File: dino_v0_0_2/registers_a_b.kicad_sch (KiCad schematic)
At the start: 8 parts, among them U31 74LS373, U32 74LS373, U33 74LS373, U35 74LS373, U41 74LS245, U42 74LS245, U43 74LS245, U44 74LS245

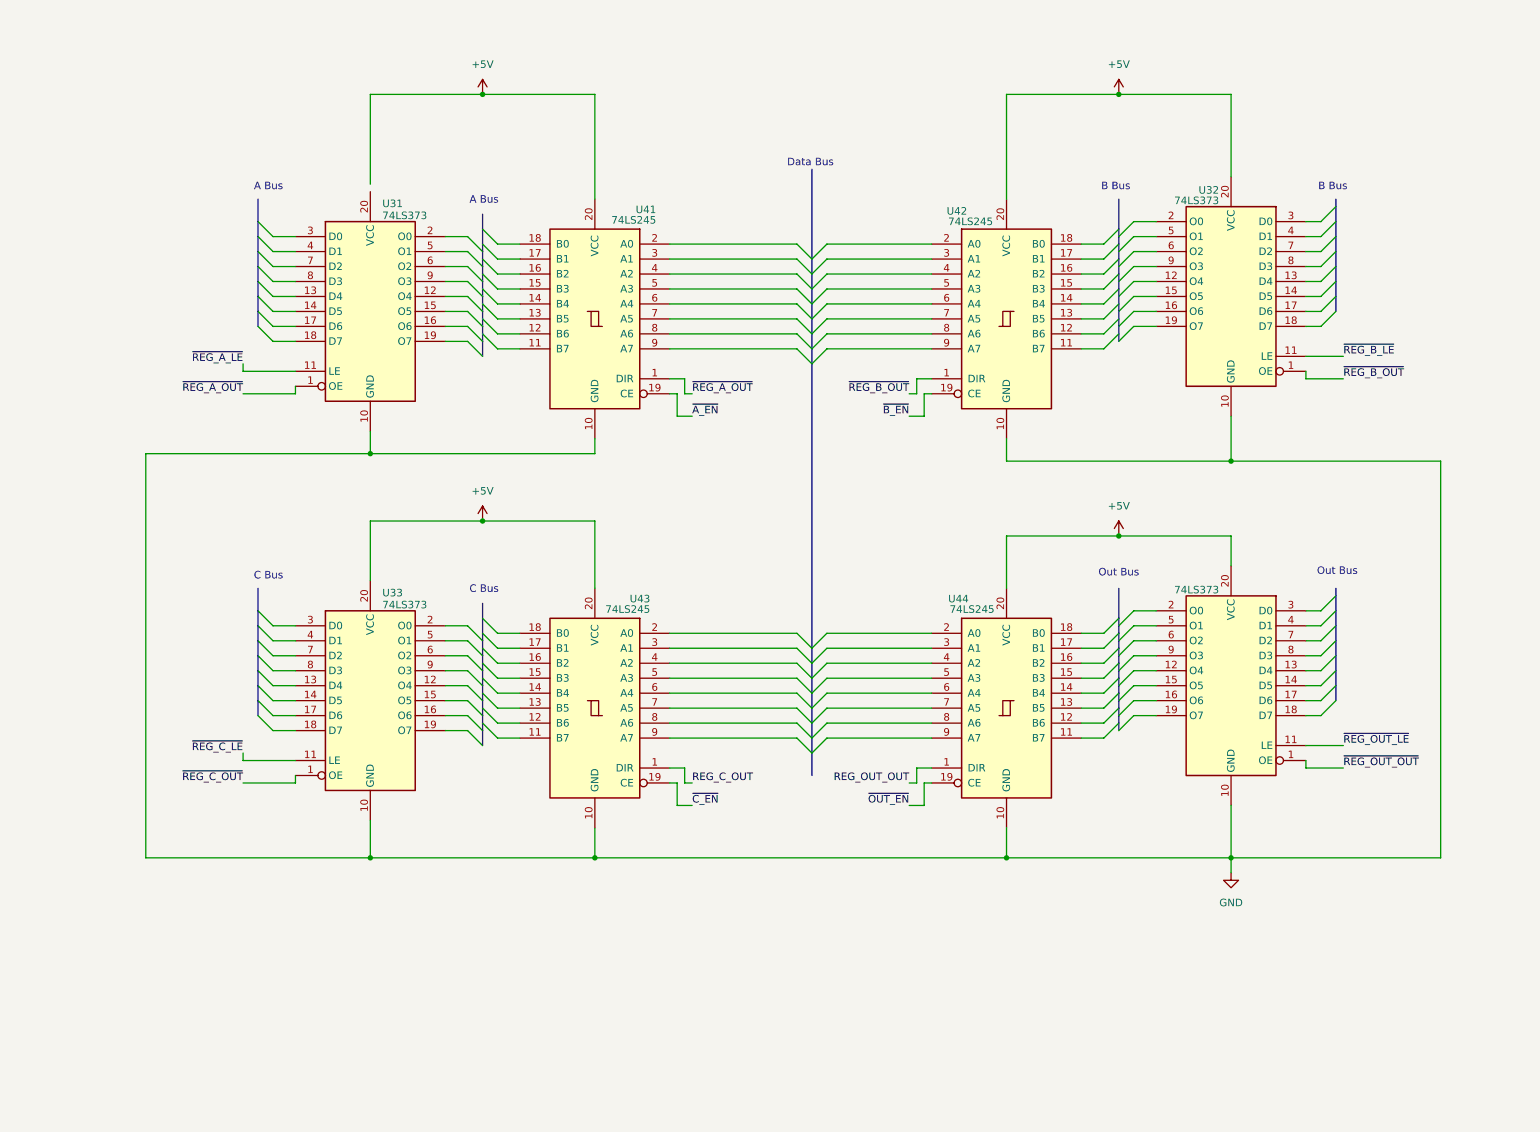
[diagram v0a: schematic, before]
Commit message: v0.3.0 - Rev 1.2.0 Update
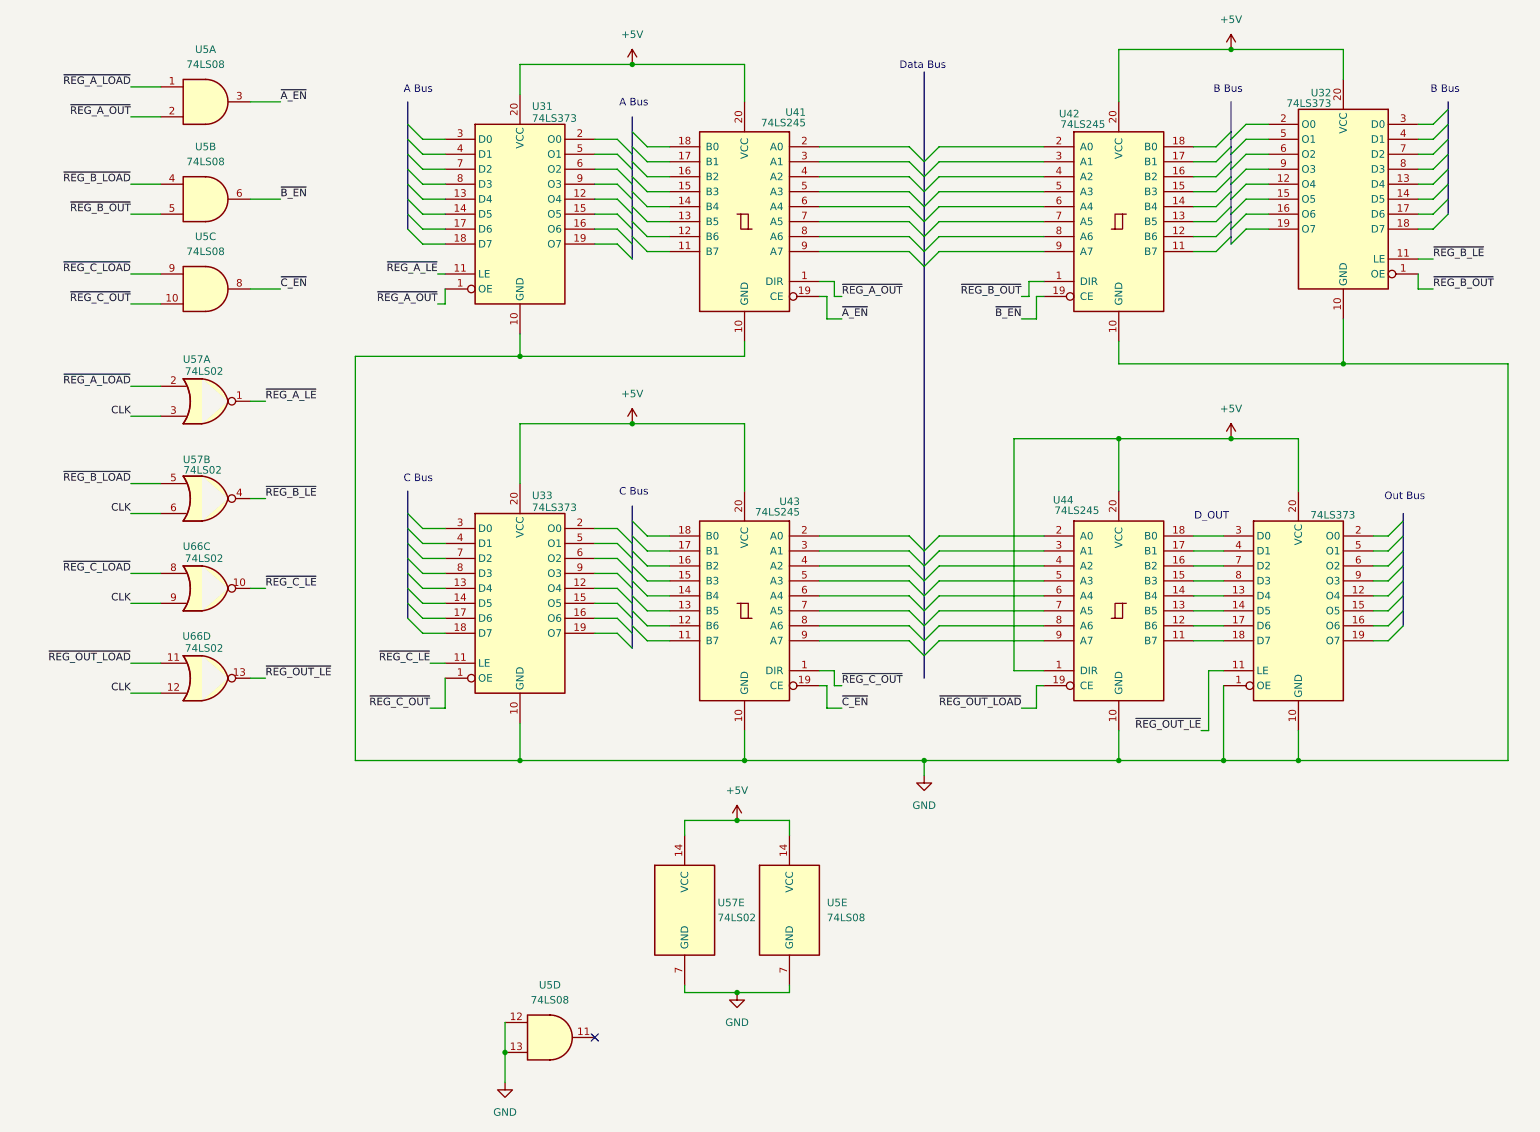
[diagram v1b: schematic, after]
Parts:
- added U5: 74LS08, symbol 74xx:74LS08
- added U57, U66: 74LS02, symbol 74xx:74LS02
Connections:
- net REG_C_OUT is gone; now on net ~{REG_C_OUT}: U43.1 (DIR)
- net REG_OUT_OUT is gone; now on net +5V: U44.1 (DIR)
- net ~{REG_OUT_OUT} is gone; now on net GND: U35.1 (OE)
- net +5V: now also U31.20 (VCC), U5.14 (VCC), U57.14 (VCC)
- net GND: now also U5.12, U5.13, U5.7 (GND), U57.7 (GND)
- net ~{A_EN}: now also U5.3
- net ~{B_EN}: now also U5.6
- net ~{C_EN}: now also U5.8
- net ~{REG_A_LE}: now also U57.1
- net ~{REG_A_OUT}: now also U5.2
- net ~{REG_B_LE}: now also U57.4
- net ~{REG_B_OUT}: now also U5.5
- net ~{REG_C_LE}: now also U66.10
- net ~{REG_C_OUT}: now also U5.10
- net ~{REG_OUT_LE}: now also U66.13
- net at U35.13 (D4): now also U44.14 (B4)
- net at U35.14 (D5): now also U44.13 (B5)
- net at U35.17 (D6): now also U44.12 (B6)
- net at U35.18 (D7): now also U44.11 (B7)
- net at U35.3 (D0): now also U44.18 (B0)
- net at U35.4 (D1): now also U44.17 (B1)
- net at U35.7 (D2): now also U44.16 (B2)
- net at U35.8 (D3): now also U44.15 (B3)
- net ~{OUT_EN} renamed ~{REG_OUT_LOAD}
- net ~{REG_OUT_LOAD}: now also U66.11
- new net CLK: U57.3, U57.6, U66.12, U66.9
- new net ~{REG_A_LOAD}: U5.1, U57.2
- new net ~{REG_B_LOAD}: U5.4, U57.5
- new net ~{REG_C_LOAD}: U5.9, U66.8
- no-connect marks 0 -> 1
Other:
- note added: "D_OUT"
- title: Dino v0.0.2 -> Dino v0.0.3
- moved on the sheet: U31, U32, U33, U41, U42, U43, U44
